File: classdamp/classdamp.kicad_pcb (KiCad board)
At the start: 2 copper layers, 46 parts, among them J2 Conn_01x02_Pin

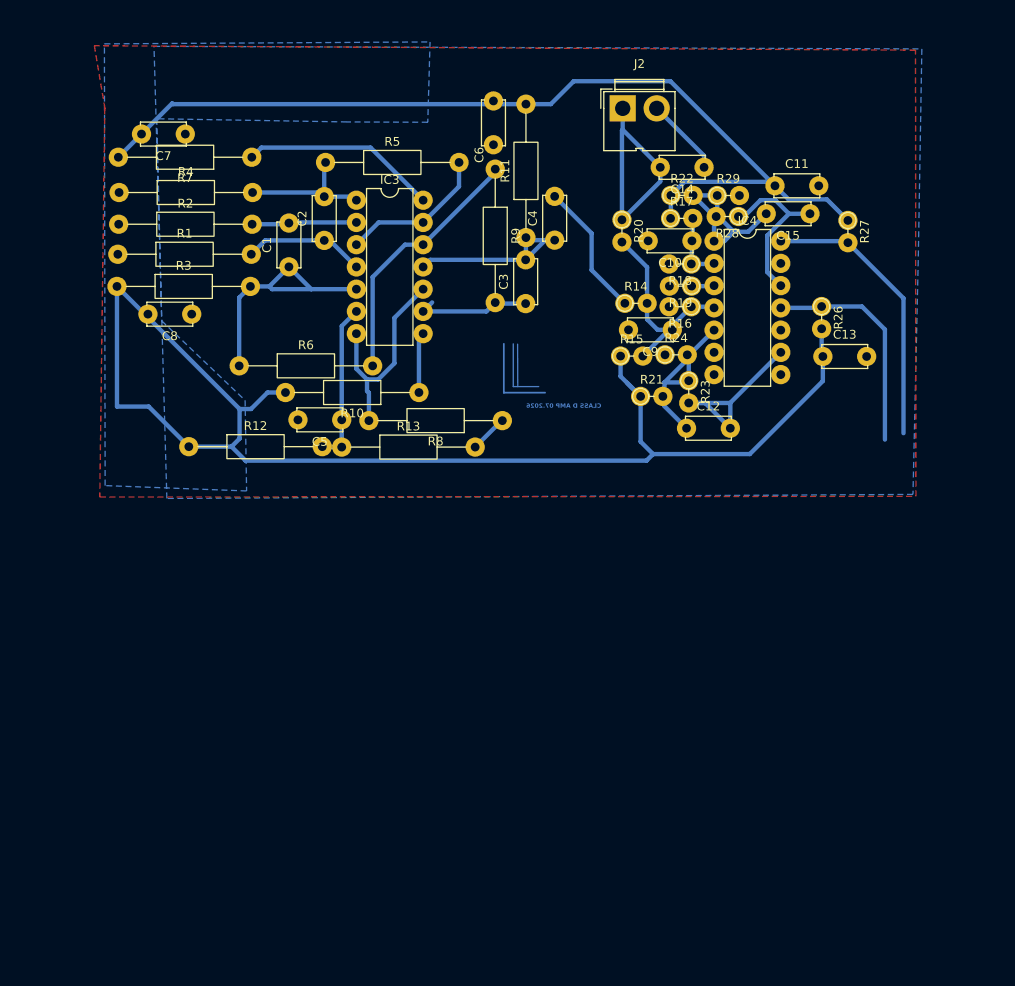
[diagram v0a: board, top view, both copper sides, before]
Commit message: PCB design done
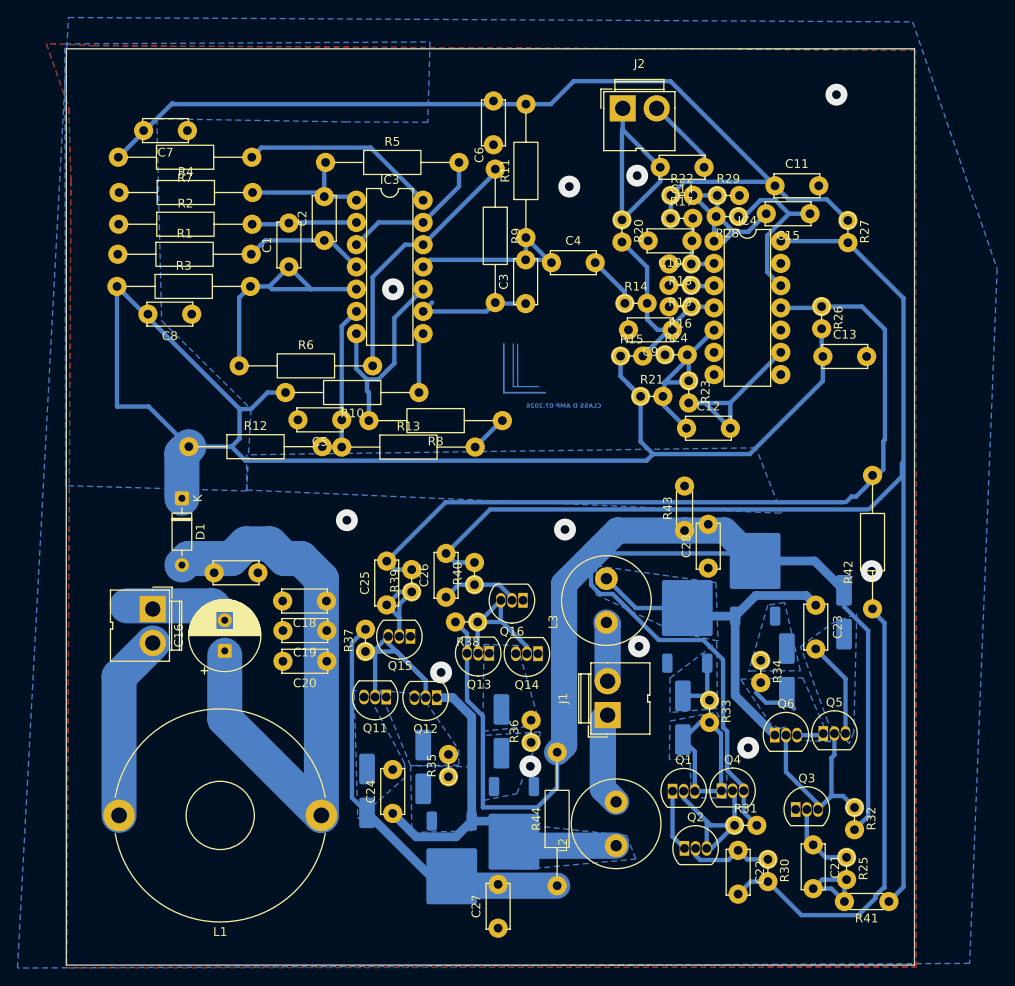
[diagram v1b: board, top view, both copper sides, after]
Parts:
- added C16: 1000u, Capacitor_THT:CP_Radial_D8.0mm_P3.50mm, F.Cu at (87.7, 129.2)
- added C17: 100n, Capacitor_THT:C_Disc_D5.0mm_W2.5mm_P5.00mm, F.Cu at (86.4, 120.3)
- added C18: 100n, Capacitor_THT:C_Disc_D5.0mm_W2.5mm_P5.00mm, F.Cu at (99.3, 123.5)
- added C19: 100n, Capacitor_THT:C_Disc_D5.0mm_W2.5mm_P5.00mm, F.Cu at (99.3, 126.9)
- added C20: 100n, Capacitor_THT:C_Disc_D5.0mm_W2.5mm_P5.00mm, F.Cu at (99.3, 130.4)
- added C21: 1n, Capacitor_THT:C_Disc_D5.0mm_W2.5mm_P5.00mm, F.Cu at (154.8, 151.4)
- added C22: 1n, Capacitor_THT:C_Disc_D5.0mm_W2.5mm_P5.00mm, F.Cu at (146.3, 152.0)
- added C23: 100n, Capacitor_THT:C_Disc_D5.0mm_W2.5mm_P5.00mm, F.Cu at (155.1, 124.0)
- added C24: 100n, Capacitor_THT:C_Disc_D5.0mm_W2.5mm_P5.00mm, F.Cu at (106.8, 147.8)
- added C25: 1n, Capacitor_THT:C_Disc_D5.0mm_W2.5mm_P5.00mm, F.Cu at (106.1, 124.0)
- added C26: 1n, Capacitor_THT:C_Disc_D5.0mm_W2.5mm_P5.00mm, F.Cu at (112.9, 123.1)
- added C27: 100n, Capacitor_THT:C_Disc_D5.0mm_W2.5mm_P5.00mm, F.Cu at (118.9, 160.9)
- added C28: 100n, Capacitor_THT:C_Disc_D5.0mm_W2.5mm_P5.00mm, F.Cu at (142.9, 119.8)
- added D1: 1N5822, Diode_THT:D_DO-35_SOD27_P7.62mm_Horizontal, F.Cu at (82.8, 111.8)
- added D2: SS14, Diode_SMD:D_SMA_Handsoldering, B.Cu at (158.4, 124.8)
- added D3: SS14, Diode_SMD:D_SMA_Handsoldering, B.Cu at (151.8, 131.5)
- added D4: SS14, Diode_SMD:D_SMA_Handsoldering, B.Cu at (140.0, 136.8)
- added D5: SS14, Diode_SMD:D_SMA_Handsoldering, B.Cu at (103.9, 145.2)
- added D6: SS14, Diode_SMD:D_SMA_Handsoldering, B.Cu at (110.3, 142.5)
- added D7: SS14, Diode_SMD:D_SMA_Handsoldering, B.Cu at (119.2, 138.4)
- added J1: Conn_01x02_Pin, Connector:JWT_A3963_1x02_P3.96mm_Vertical, F.Cu at (131.4, 136.6)
- added J3: Conn_01x02_Pin, Connector:JWT_A3963_1x02_P3.96mm_Vertical, F.Cu at (79.4, 124.4)
- added L1: 100u, Inductor_THT:L_Toroid_Horizontal_D24.1mm_P23.10mm_Bourns_2200, F.Cu at (98.7, 148.0)
- added L2: 15u, Inductor_THT:L_Radial_D10.0mm_P5.00mm_Fastron_07M, F.Cu at (132.3, 151.5)
- added L3: 15u, Inductor_THT:L_Radial_D10.0mm_P5.00mm_Fastron_07M, F.Cu at (131.2, 126.0)
- added Q1: S8550, Package_TO_SOT_THT:TO-92_Inline, F.Cu at (138.8, 145.2)
- added Q10: IPD135N03LGATMA1, Package_TO_SOT_SMD:TO-252-2, B.Cu at (120.7, 149.7)
- added Q11: S8050, Package_TO_SOT_THT:TO-92_Inline, F.Cu at (106.1, 134.5)
- added Q12: S8550, Package_TO_SOT_THT:TO-92_Inline, F.Cu at (111.9, 134.6)
- added Q13: S8050, Package_TO_SOT_THT:TO-92_Inline, F.Cu at (117.9, 129.5)
- added Q14: S8550, Package_TO_SOT_THT:TO-92_Inline, F.Cu at (123.4, 129.5)
- added Q15: 2N5551, Package_TO_SOT_THT:TO-92_Inline, F.Cu at (108.9, 127.6)
- added Q16: 2N5551, Package_TO_SOT_THT:TO-92_Inline, F.Cu at (121.7, 123.4)
- added Q2: 2N5551, Package_TO_SOT_THT:TO-92_Inline, F.Cu at (140.1, 151.8)
- added Q3: 2N5551, Package_TO_SOT_THT:TO-92_Inline, F.Cu at (152.9, 147.3)
- added Q4: S8050, Package_TO_SOT_THT:TO-92_Inline, F.Cu at (144.4, 145.2)
- added Q5: S8050, Package_TO_SOT_THT:TO-92_Inline, F.Cu at (156.0, 138.7)
- added Q6: S8550, Package_TO_SOT_THT:TO-92_Inline, F.Cu at (150.5, 138.8)
- added Q7: IPD135N03LGATMA1, Package_TO_SOT_SMD:TO-252-2, B.Cu at (140.5, 125.6)
- added Q8: IPD135N03LGATMA1, Package_TO_SOT_SMD:TO-252-2, B.Cu at (148.2, 120.2)
- added Q9: IPD135N03LGATMA1, Package_TO_SOT_SMD:TO-252-2, B.Cu at (113.6, 153.7)
- added R25: 10k, Library:R_Axial_DIN0204_L3.6mm_D1.6mm_P2.54mm_Vertical, F.Cu at (158.7, 152.8)
- added R30: 10k, Library:R_Axial_DIN0204_L3.6mm_D1.6mm_P2.54mm_Vertical, F.Cu at (149.7, 153.0)
- added R31: 1k, Library:R_Axial_DIN0204_L3.6mm_D1.6mm_P2.54mm_Vertical, F.Cu at (145.9, 149.1)
- added R32: 1k, Library:R_Axial_DIN0204_L3.6mm_D1.6mm_P2.54mm_Vertical, F.Cu at (159.6, 147.1)
- added R33: 150, Library:R_Axial_DIN0204_L3.6mm_D1.6mm_P2.54mm_Vertical, F.Cu at (143.0, 134.9)
- added R34: 200, Library:R_Axial_DIN0204_L3.6mm_D1.6mm_P2.54mm_Vertical, F.Cu at (148.9, 130.3)
- added R35: 200, Library:R_Axial_DIN0204_L3.6mm_D1.6mm_P2.54mm_Vertical, F.Cu at (113.2, 143.6)
- added R36: 150, Library:R_Axial_DIN0204_L3.6mm_D1.6mm_P2.54mm_Vertical, F.Cu at (122.6, 139.7)
- added R37: 1k, Library:R_Axial_DIN0204_L3.6mm_D1.6mm_P2.54mm_Vertical, F.Cu at (103.7, 129.3)
- added R38: 1k, Library:R_Axial_DIN0204_L3.6mm_D1.6mm_P2.54mm_Vertical, F.Cu at (116.5, 125.9)
- added R39: 10k, Library:R_Axial_DIN0204_L3.6mm_D1.6mm_P2.54mm_Vertical, F.Cu at (109.0, 122.5)
- added R40: 10k, Library:R_Axial_DIN0204_L3.6mm_D1.6mm_P2.54mm_Vertical, F.Cu at (116.2, 121.7)
- added R41: 0, Resistor_THT:R_Axial_DIN0204_L3.6mm_D1.6mm_P5.08mm_Horizontal, F.Cu at (163.5, 157.8)
- added R42: 0, Resistor_THT:R_Axial_DIN0207_L6.3mm_D2.5mm_P15.24mm_Horizontal, F.Cu at (161.6, 124.4)
- added R43: 0, Resistor_THT:R_Axial_DIN0204_L3.6mm_D1.6mm_P5.08mm_Horizontal, F.Cu at (140.2, 115.5)
- added R44: 0, Resistor_THT:R_Axial_DIN0207_L6.3mm_D2.5mm_P15.24mm_Horizontal, F.Cu at (125.6, 156.0)
- R8: value 1k -> 330
- R9: value 47k -> 50k
- moved C4 2.60 mm to (125.0, 84.9), turned to 0 degrees
- moved C7 0.46 mm to (83.4, 69.8)
- moved R19 0.10 mm to (140.9, 87.5)
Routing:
- net +12V: track 259.9 -> 496.2 mm
- net Net-(IC4-Q5_C): track 32.1 -> 158.0 mm
- net Net-(IC4-Q4_C): track 25.9 -> 146.2 mm
- net Net-(D1-A): track 0.00 -> 68.5 mm
- net PRI2_MID: track 0.00 -> 45.3 mm
- net PRI_MID: track 0.00 -> 42.6 mm
- net Net-(Q11-B): track 0.00 -> 24.6 mm
- net Net-(Q3-C): track 0.00 -> 22.6 mm
- net Net-(D4-K): track 0.00 -> 21.8 mm
- net +12VA: track 0.00 -> 21.3 mm
- net Net-(Q1-B): track 0.00 -> 19.3 mm
- net GND: track 31.0 -> 49.8 mm, vias 0 -> 11
- net Net-(Q13-B): track 0.00 -> 17.4 mm
- net Net-(Q15-B): track 0.00 -> 11.2 mm
- net PRI_HI: track 0.00 -> 11.1 mm
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- added copper zone on B.Cu, net Net-(D3-A)
- added copper zone on B.Cu, net Net-(D3-K)
- added copper zone on B.Cu, net Net-(D4-A)
- added copper zone on B.Cu, net Net-(D4-K)
- added copper zone on B.Cu, net Net-(D6-A)
- added copper zone on B.Cu, net Net-(D6-K)
- added copper zone on B.Cu, net Net-(D7-A)
- added copper zone on B.Cu, net Net-(D7-K)
- added copper zone on B.Cu, net PRI2_HI
- added copper zone on B.Cu, net PRI2_MID
- added copper zone on B.Cu, net PRI_HI
- added copper zone on B.Cu, net PRI_MID
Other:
- board outline added: 96.9 x 104.6 mm
